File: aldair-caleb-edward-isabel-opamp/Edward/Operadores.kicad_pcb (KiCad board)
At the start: 2 copper layers, 190.2 x 71.5 mm, 50 parts, among them J1 Conn_01x01_Pin, J10 Conn_01x01_Pin, J11 Conn_01x01_Pin, J12 Conn_01x01_Pin, J13 Conn_01x01_Pin, J14 Conn_01x01_Pin, J15 Conn_01x01_Pin, J16 Conn_01x01_Pin, J2 Conn_01x01_Pin, J3 Conn_01x01_Pin, J4 Conn_01x01_Pin, J5 Conn_01x01_Pin, J6 Conn_01x01_Pin, J7 Conn_01x01_Pin, J8 Conn_01x01_Pin, J9 Conn_01x01_Pin, U1 LM741, U2 LM741, U3 LM741, U4 LM741, U5 LM741, U6 LM741, U7 LM741, U8 LM741

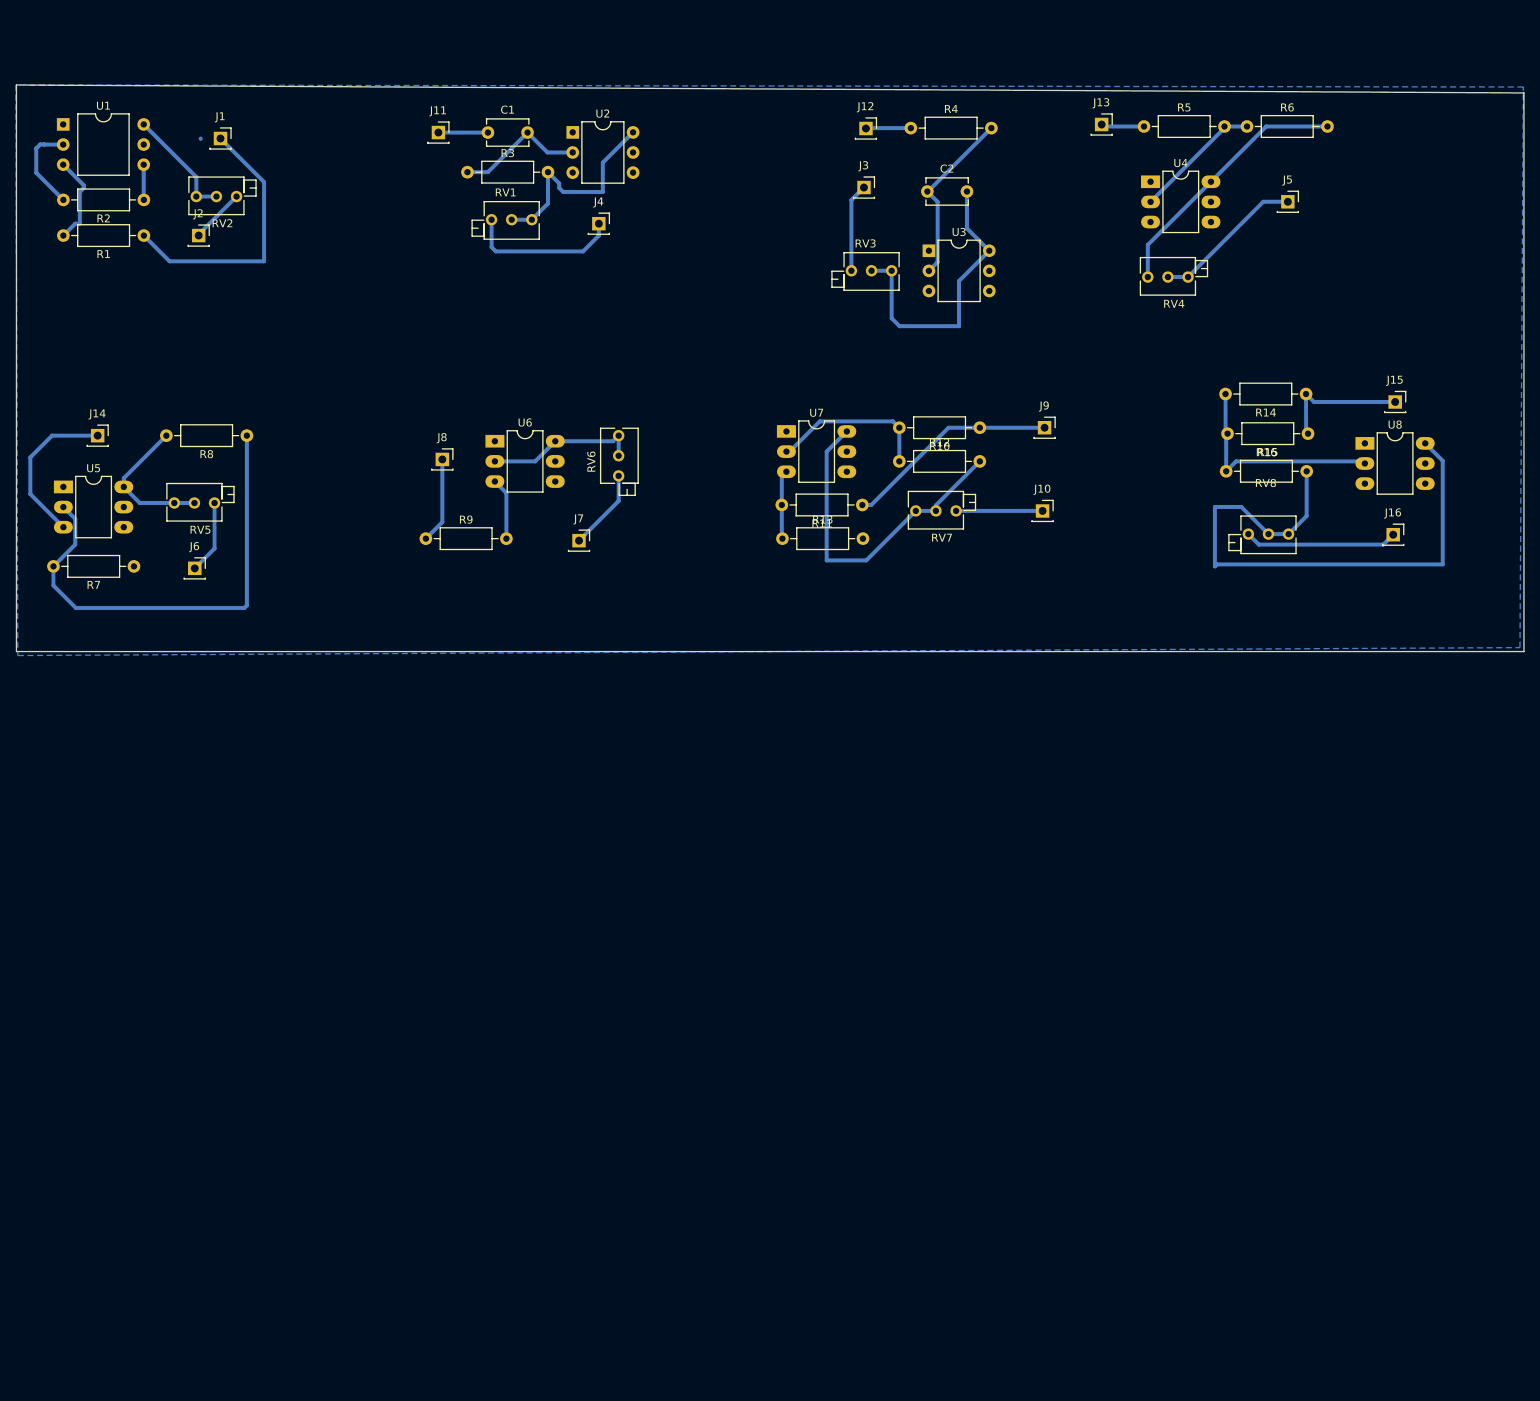
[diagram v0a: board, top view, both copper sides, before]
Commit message: Cambios Finales Prueba OP AMP - EDWARDS
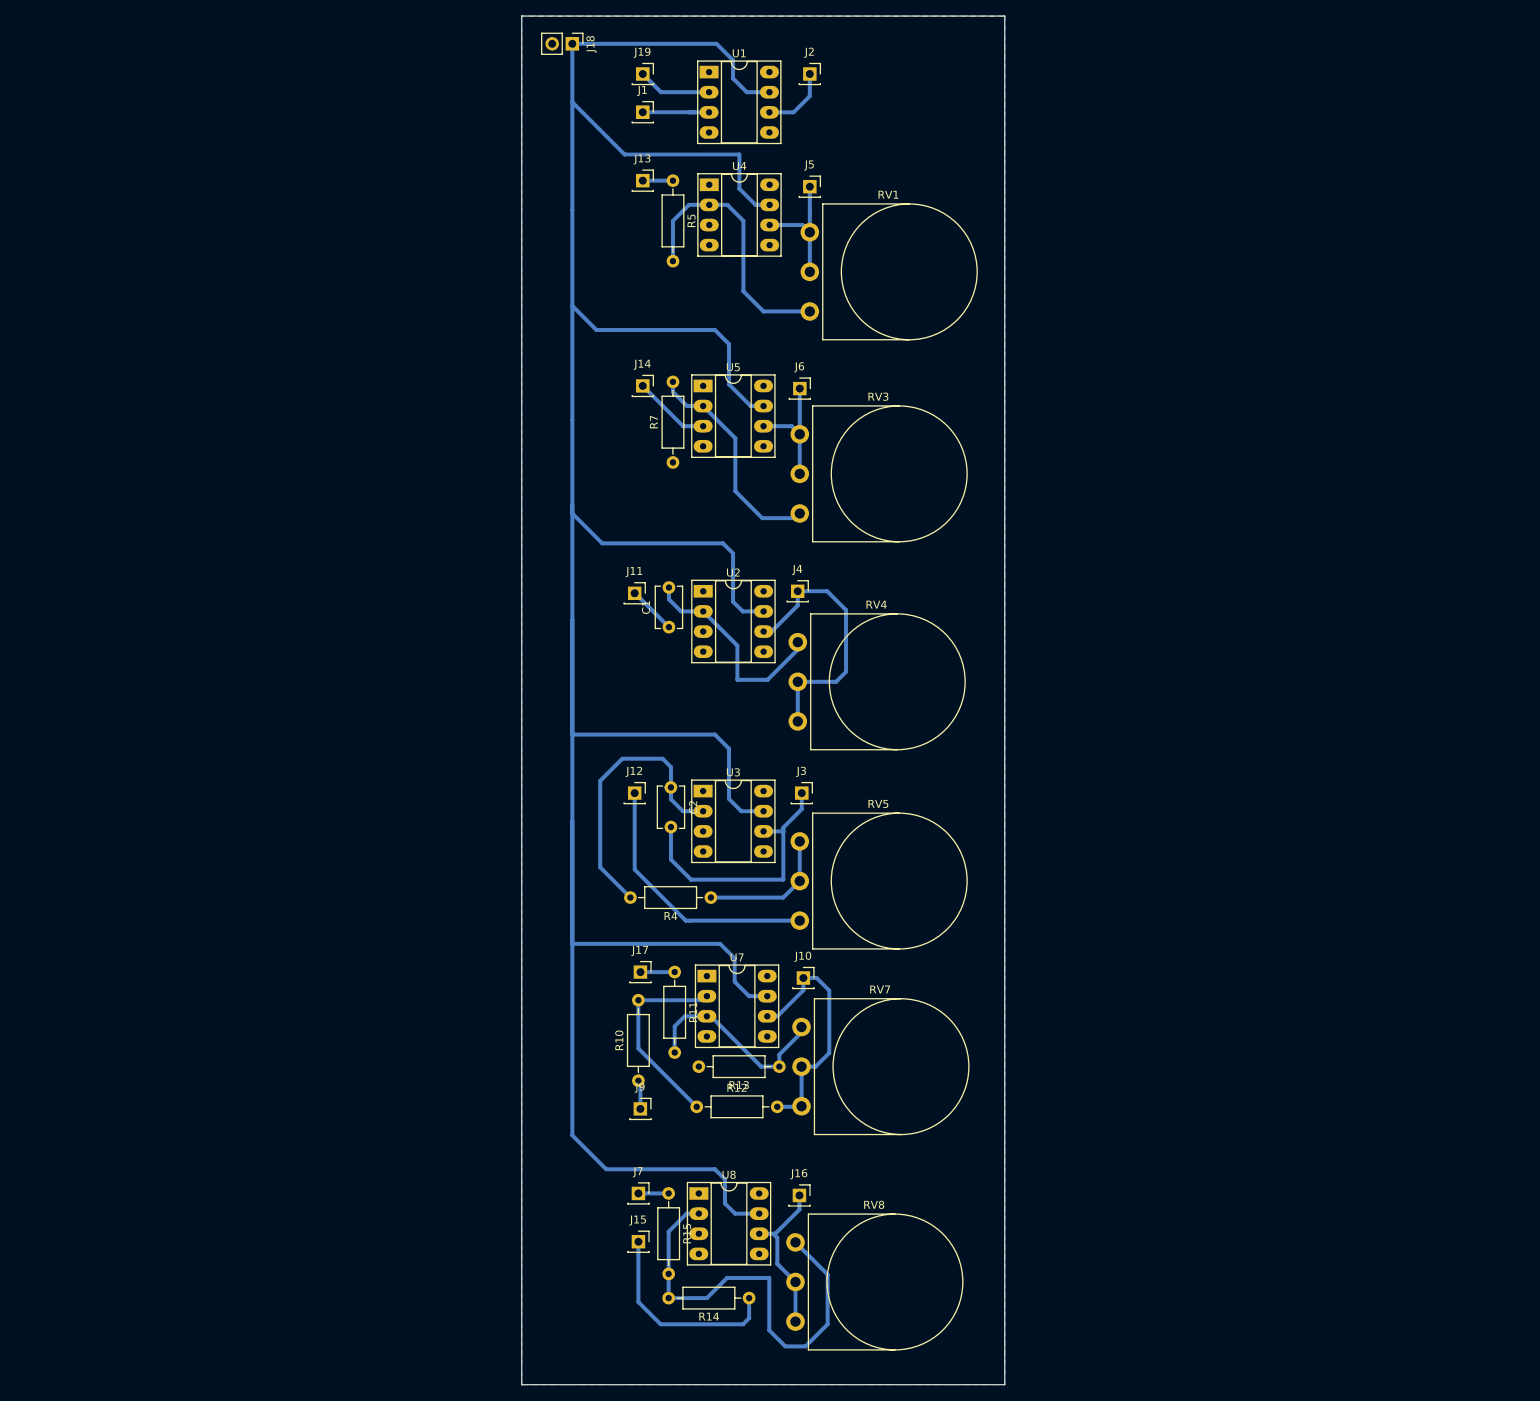
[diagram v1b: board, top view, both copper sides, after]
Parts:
- removed J8: Conn_01x01_Pin, Connector_PinSocket_2.54mm:PinSocket_1x01_P2.54mm_Vertical
- removed R1, R16, R2, R3, R6, R8, R9: R, Resistor_THT:R_Axial_DIN0207_L6.3mm_D2.5mm_P10.16mm_Horizontal
- removed RV2, RV6: R_Potentiometer, Potentiometer_THT:Potentiometer_Bourns_3266Z_Horizontal
- removed U6: LM741, Package_DIP:DIP-6_W7.62mm_LongPads
- added J17: Conn_01x01_Pin, Connector_PinSocket_2.54mm:PinSocket_1x01_P2.54mm_Vertical, F.Cu at (111.3, 139.5)
- added J18: Conn_01x02_Pin, Connector_PinHeader_2.54mm:PinHeader_1x02_P2.54mm_Vertical, F.Cu at (102.7, 22.3)
- added J19: Conn_01x01_Pin, Connector_PinSocket_2.54mm:PinSocket_1x01_P2.54mm_Vertical, F.Cu at (111.5, 26.1)
- RV1, RV3, RV4, RV5, RV7, RV8: footprint Potentiometer_THT:Potentiometer_Bourns_3266Z_Horizontal -> Potentiometer_THT:Potentiometer_Omeg_PC16BU_Vertical
- U1: footprint Package_DIP:DIP-6_W10.16mm -> Package_DIP:DIP-8_W7.62mm_Socket_LongPads
- U2, U3: footprint Package_DIP:DIP-6_W7.62mm -> Package_DIP:DIP-8_W7.62mm_Socket_LongPads
- U4, U5, U7, U8: footprint Package_DIP:DIP-6_W7.62mm_LongPads -> Package_DIP:DIP-8_W7.62mm_Socket_LongPads
- moved J15 142.7 mm to (111.0, 173.5)
- moved R14 134.0 mm to (125.0, 180.6)
- moved U8 126.6 mm to (118.6, 167.4)
- moved R15 125.3 mm to (114.8, 167.4), turned to -90 degrees
- moved RV8 117.3 mm to (130.8, 183.6)
- moved J16 112.1 mm to (131.3, 167.6)
- moved R4 100.3 mm to (120.1, 130.0), turned to 180 degrees
- moved J9 100.0 mm to (111.2, 156.7)
- moved RV5 94.9 mm to (131.4, 133.0), turned to 0 degrees
- moved R10 93.0 mm to (111.0, 153.2), turned to 90 degrees
- moved J12 88.8 mm to (110.5, 116.9)
- moved R12 85.4 mm to (118.4, 156.5)
- moved J7 82.7 mm to (111.0, 167.4)
- moved C2 81.9 mm to (115.1, 116.1), turned to -90 degrees
- moved U1 81.8 mm to (119.9, 25.9)
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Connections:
- C2 pad 2: Net-(C2-Pad2) -> Net-(J3-Pin_1)
- R11 pad 1: Net-(J9-Pin_1) -> Net-(J17-Pin_1)
- R12 pad 2: Net-(R12-Pad2) -> Net-(J10-Pin_1)
- R15 pad 1: Net-(J15-Pin_1) -> Net-(J7-Pin_1)
- R4 pad 1: Net-(J12-Pin_1) -> Net-(R4-Pad1)
- RV1 pad 1: Net-(R3-Pad2) -> Net-(U4--)
- RV1 pad 2: Net-(R3-Pad2) -> Net-(J5-Pin_1)
- RV1 pad 3: Net-(J4-Pin_1) -> Net-(J5-Pin_1)
- RV3 pad 1: Net-(C2-Pad2) -> Net-(U5--)
- RV3 pad 2: Net-(C2-Pad2) -> Net-(J6-Pin_1)
- RV3 pad 3: Net-(J3-Pin_1) -> Net-(J6-Pin_1)
- RV4 pad 1: Net-(R6-Pad2) -> Net-(J4-Pin_1)
- RV4 pad 2: Net-(J5-Pin_1) -> Net-(J4-Pin_1)
- RV4 pad 3: Net-(J5-Pin_1) -> Net-(U2--)
- RV5 pad 1: Net-(R8-Pad2) -> Net-(J12-Pin_1)
- RV5 pad 2: Net-(R8-Pad2) -> Net-(R4-Pad1)
- RV5 pad 3: Net-(J6-Pin_1) -> Net-(R4-Pad1)
- RV7 pad 1: Net-(R12-Pad2) -> Net-(J10-Pin_1)
- RV7 pad 2: Net-(R12-Pad2) -> Net-(J10-Pin_1)
- RV7 pad 3: Net-(J10-Pin_1) -> Net-(U7-+)
- RV8 pad 1: Net-(R16-Pad2) -> Net-(J16-Pin_1)
- RV8 pad 2: Net-(R16-Pad2) -> Net-(J16-Pin_1)
- RV8 pad 3: Net-(J16-Pin_1) -> Net-(U8--)
- U1 pad 3: Net-(U1-+) -> Net-(J1-Pin_1)
- U1 pad 6: Net-(RV2-Pad1) -> Net-(J2-Pin_1)
- U2 pad 6: Net-(R3-Pad2) -> Net-(J4-Pin_1)
- U3 pad 6: Net-(C2-Pad2) -> Net-(J3-Pin_1)
- U4 pad 6: Net-(R6-Pad2) -> Net-(J5-Pin_1)
- U5 pad 6: Net-(R8-Pad2) -> Net-(J6-Pin_1)
- U7 pad 6: Net-(R12-Pad2) -> Net-(J10-Pin_1)
- U8 pad 6: Net-(R16-Pad2) -> Net-(J16-Pin_1)
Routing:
- net VCC: track 0.00 -> 385.9 mm
- net Net-(R16-Pad2): track 72.1 -> 0.00 mm
- net Net-(R12-Pad2): track 42.3 -> 0.00 mm
- net Net-(C2-Pad2): track 37.2 -> 0.00 mm
- net Net-(R6-Pad2): track 32.9 -> 0.00 mm
- net Net-(U5--): track 58.8 -> 27.5 mm
- net Net-(J12-Pin_1): track 5.69 -> 33.1 mm
- net Net-(U8--): track 28.1 -> 54.9 mm
- net Net-(R3-Pad2): track 26.8 -> 0.00 mm
- net Net-(J1-Pin_1): track 34.3 -> 9.13 mm
- net Net-(J3-Pin_1): track 11.2 -> 34.8 mm
- net Net-(J9-Pin_1): track 27.0 -> 3.66 mm
- net Net-(J10-Pin_1): track 10.9 -> 31.6 mm
- net Net-(U6--): track 19.5 -> 0.00 mm
- net Net-(R8-Pad2): track 18.5 -> 0.00 mm
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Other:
- board size 190.2 x 71.5 mm -> 61 x 172.7 mm
